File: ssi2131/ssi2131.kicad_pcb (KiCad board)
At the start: 2 copper layers, 40.2 x 108 mm, 34 parts, among them J1 Saw Out, J2 Pulse Out, J3 Tri Out, J4 Hard Sync, J5 Soft Sync, J6 Expo Freq, J7 16-Pin uZeus Power Header, U1 SSI2131, U2 LM4040DBZ-2.5

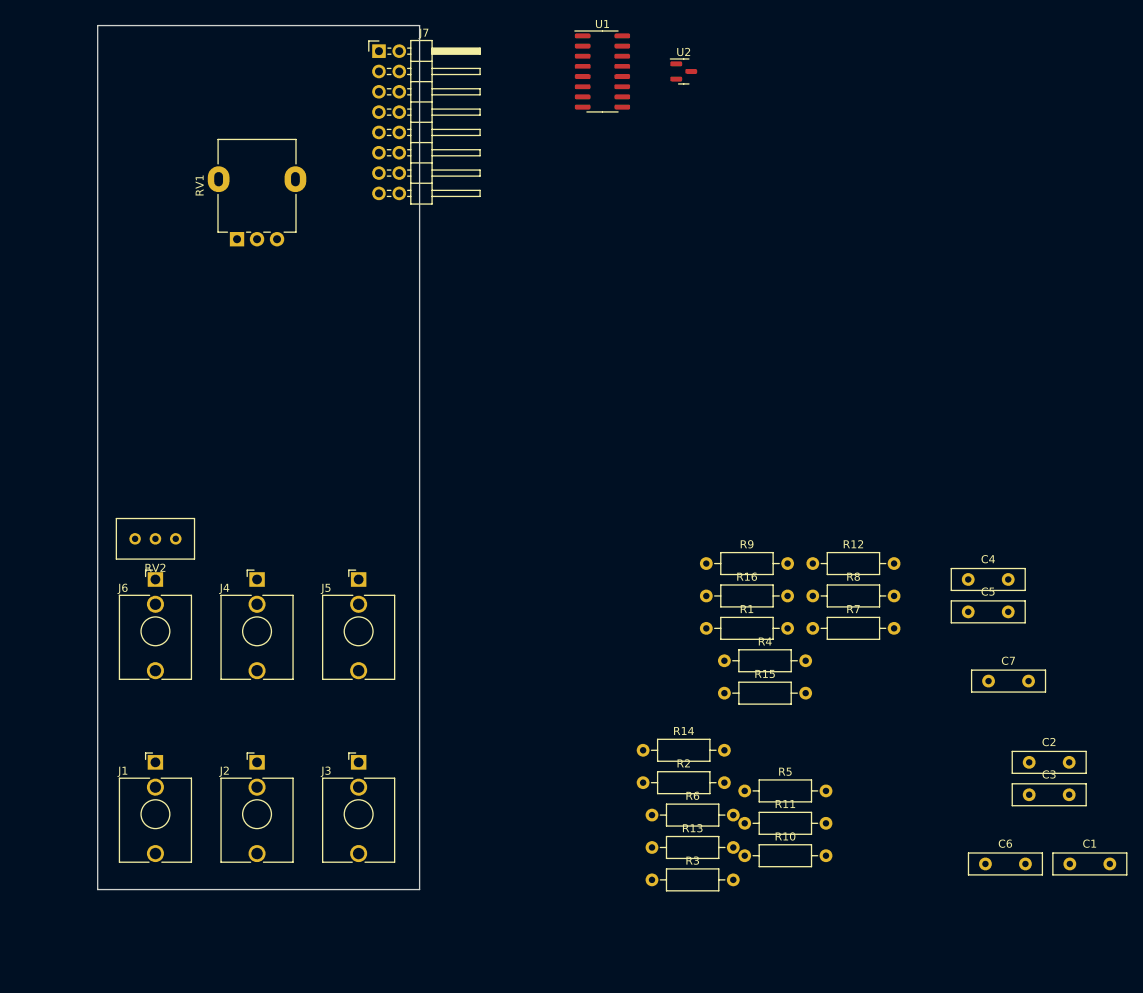
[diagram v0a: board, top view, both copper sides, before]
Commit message: PCB attempt 1
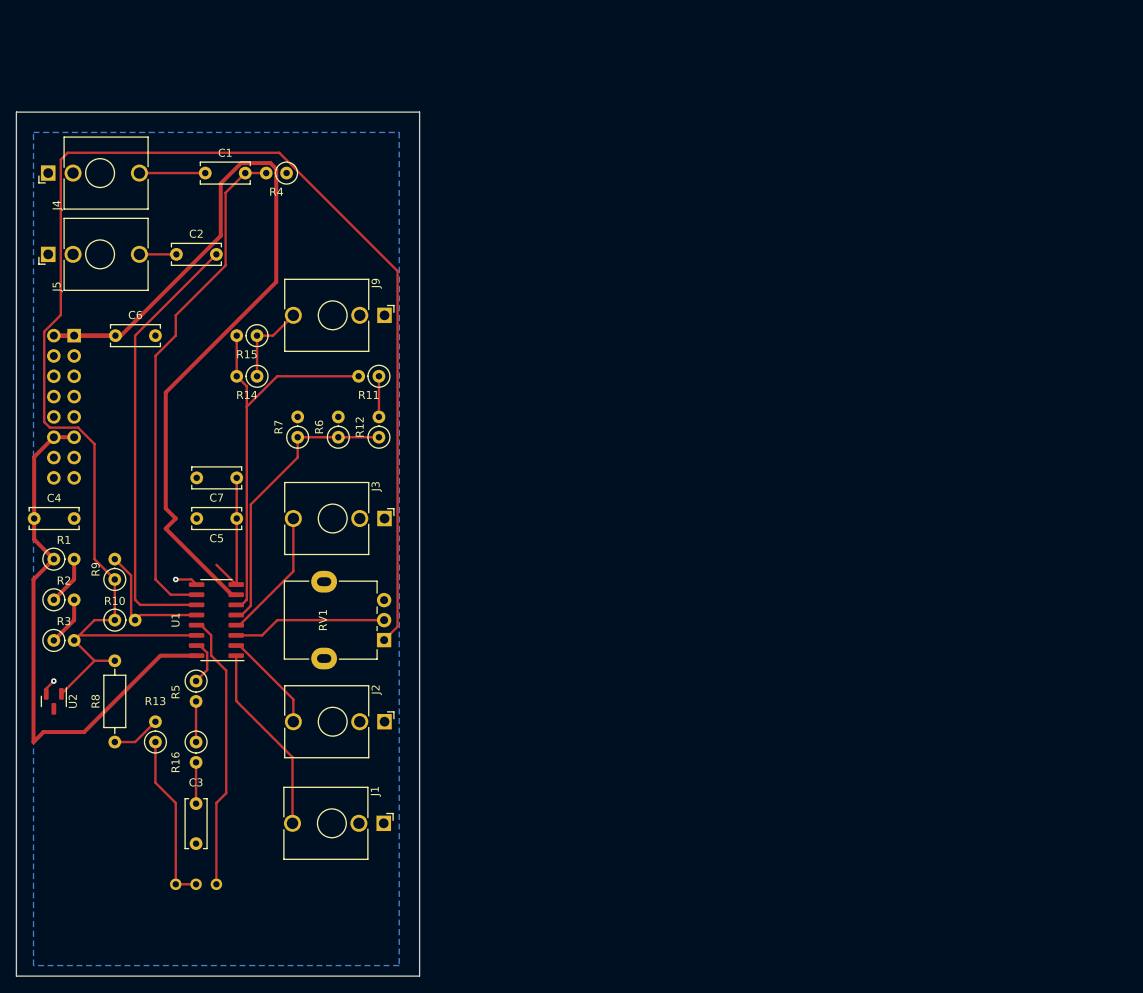
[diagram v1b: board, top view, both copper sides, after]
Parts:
- removed J6: Expo Freq, Connector_Audio:Jack_3.5mm_QingPu_WQP-PJ398SM_Vertical_CircularHoles
- added J9: Expo Freq, Connector_Audio:Jack_3.5mm_QingPu_WQP-PJ398SM_Vertical_CircularHoles, F.Cu at (135.3, 55.9)
- C1, C2, C3, C4, C5, C6, C7: footprint Capacitor_THT:C_Disc_D9.0mm_W2.5mm_P5.00mm -> Capacitor_THT:C_Disc_D6.0mm_W2.5mm_P5.00mm
- J7: footprint Connector_PinHeader_2.54mm:PinHeader_2x08_P2.54mm_Horizontal -> Connector_PinHeader_2.54mm:PinHeader_2x08_P2.54mm_Vertical; moved to B.Cu
- R1, R10, R13, R16, R2, R3, R4, R5, R6, R7, R9: footprint Resistor_THT:R_Axial_DIN0207_L6.3mm_D2.5mm_P10.16mm_Horizontal -> Resistor_THT:R_Axial_DIN0207_L6.3mm_D2.5mm_P2.54mm_Vertical
- R11: value 100 kOhms -> 220 kOhms; footprint Resistor_THT:R_Axial_DIN0207_L6.3mm_D2.5mm_P10.16mm_Horizontal -> Resistor_THT:R_Axial_DIN0207_L6.3mm_D2.5mm_P2.54mm_Vertical
- R12: value 100 kOhms -> 47 kOhms; footprint Resistor_THT:R_Axial_DIN0207_L6.3mm_D2.5mm_P10.16mm_Horizontal -> Resistor_THT:R_Axial_DIN0207_L6.3mm_D2.5mm_P2.54mm_Vertical
- R14: value 220 kOhms -> 100 kOhms; footprint Resistor_THT:R_Axial_DIN0207_L6.3mm_D2.5mm_P10.16mm_Horizontal -> Resistor_THT:R_Axial_DIN0207_L6.3mm_D2.5mm_P2.54mm_Vertical
- R15: value 47 kOhms -> 100 kOhms; footprint Resistor_THT:R_Axial_DIN0207_L6.3mm_D2.5mm_P10.16mm_Horizontal -> Resistor_THT:R_Axial_DIN0207_L6.3mm_D2.5mm_P2.54mm_Vertical
- RV2: value Expo Scale Knob - 5 kOhms -> Expo Scale Trim - 5 kOhms; moved to B.Cu
- moved C1 138.3 mm to (112.9, 38.1)
- moved C6 123.0 mm to (106.7, 58.4), turned to 180 degrees
- moved C2 119.8 mm to (114.3, 48.3), turned to 180 degrees
- moved C4 112.0 mm to (96.5, 81.3), turned to 180 degrees
- moved U2 111.4 mm to (94.0, 104.1), turned to -90 degrees
- moved C3 104.3 mm to (111.8, 121.9), turned to 90 degrees
- moved C7 97.4 mm to (116.8, 76.2), turned to 180 degrees
- moved C5 92.2 mm to (116.8, 81.3), turned to 180 degrees
- moved R8 89.1 mm to (101.6, 109.2), turned to 90 degrees
- moved R10 84.1 mm to (101.6, 94.0)
- moved U1 83.9 mm to (114.3, 94.0), turned to 180 degrees
- moved R1 82.0 mm to (94.0, 86.4)
- moved R4 81.9 mm to (123.1, 38.1), turned to 180 degrees
- moved R3 80.5 mm to (94.0, 96.5)
- moved R2 77.1 mm to (94.0, 91.4)
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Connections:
- net +2V5 renamed VREF
- net Net-(C1-Pad2) renamed HardSync
- net Net-(C2-Pad1) renamed SoftSync
- net Net-(C5-Pad1) renamed TCAP
- net Net-(J1-PadT) renamed SawOut
- net Net-(J2-PadT) renamed PulseOut
- net Net-(J3-PadT) renamed TriOut
- net Net-(R10-Pad2) renamed LinFreq
- net Net-(R5-Pad1) renamed BWComp
- net Net-(RV1-Pad2) renamed PWMCtrl
- net Net-(RV2-Pad1) renamed ExpoScale
- J7 pad 11: unconnected-(J7-Pad11) -> +5V
- J7 pad 12: unconnected-(J7-Pad12) -> +5V
- J7 pad 2: unconnected-(J7-Pad2) -> -12V
- J7 pad 4: unconnected-(J7-Pad4) -> GND
- J7 pad 6: unconnected-(J7-Pad6) -> GND
- J7 pad 8: unconnected-(J7-Pad8) -> GND
- J7 pad 9: +5V -> unconnected-(J7-Pad9)
- R11 pad 1: Net-(J6-PadT) -> Net-(R11-Pad1)
- R11 pad 2: Net-(R11-Pad2) -> ExpoFreq
- R12 pad 1: Net-(J6-PadT) -> HFTrack
- R12 pad 2: Net-(R11-Pad2) -> Net-(R11-Pad1)
- R14 pad 1: Net-(R11-Pad2) -> Net-(J9-PadT)
- R14 pad 2: Net-(R14-Pad2) -> ExpoFreq
- R15 pad 1: Net-(R14-Pad2) -> Net-(J9-PadT)
- R15 pad 2: Net-(R15-Pad2) -> ExpoFreq
- R6 pad 1: Net-(R15-Pad2) -> HFTrack
- R7 pad 1: Net-(R15-Pad2) -> HFTrack
- U1 pad 5: Net-(R15-Pad2) -> HFTrack
- U1 pad 6: Net-(R11-Pad2) -> ExpoFreq
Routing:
- net VREF: track 0.00 -> 193.2 mm
- net -12V: track 0.00 -> 112.5 mm
- net +5V: track 0.00 -> 68.6 mm
- net HardSync: track 0.00 -> 64.0 mm
- net SoftSync: track 0.00 -> 55.3 mm
- net ExpoFreq: track 0.00 -> 50.7 mm
- net HFTrack: track 0.00 -> 36.0 mm
- net ExpoScale: track 0.00 -> 34.8 mm
- net SawOut: track 0.00 -> 23.9 mm
- net Net-(R13-Pad1): track 0.00 -> 21.4 mm
- net PWMCtrl: track 0.00 -> 19.3 mm
- net TCAP: track 0.00 -> 16.9 mm
- net LinFreq: track 0.00 -> 16.6 mm
- net TriOut: track 0.00 -> 16.5 mm
- net PulseOut: track 0.00 -> 12.7 mm
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- added copper zone on B.Cu, net GND
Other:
- board size 40.2 x 108 mm -> 50.4 x 108 mm
